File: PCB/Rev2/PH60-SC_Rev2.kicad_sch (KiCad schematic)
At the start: 43 parts, among them J1 USB_C_Receptacle_USB2.0_14P, J2 Conn_01x02_Pin, J3 Conn_01x02_Pin, U1 nRF52840, X1 32.768kHz, X2 Crystal_Generic

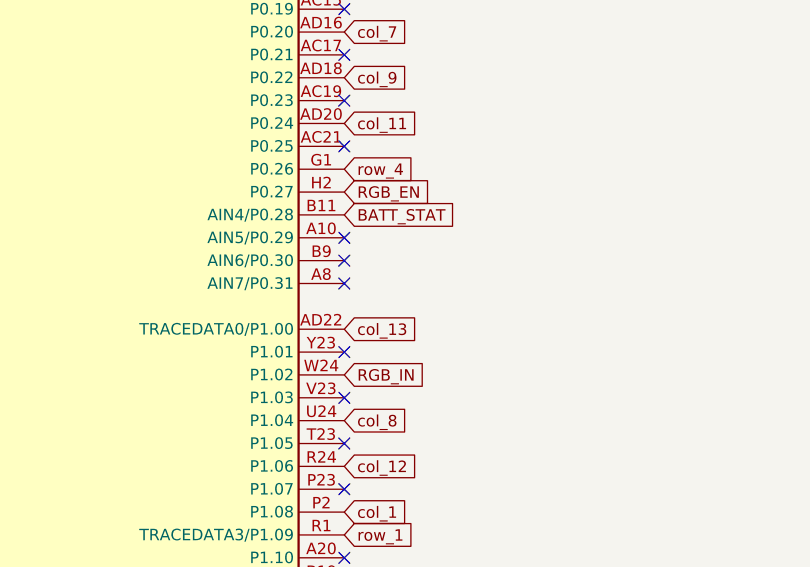
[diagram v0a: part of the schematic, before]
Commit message: layout and drc
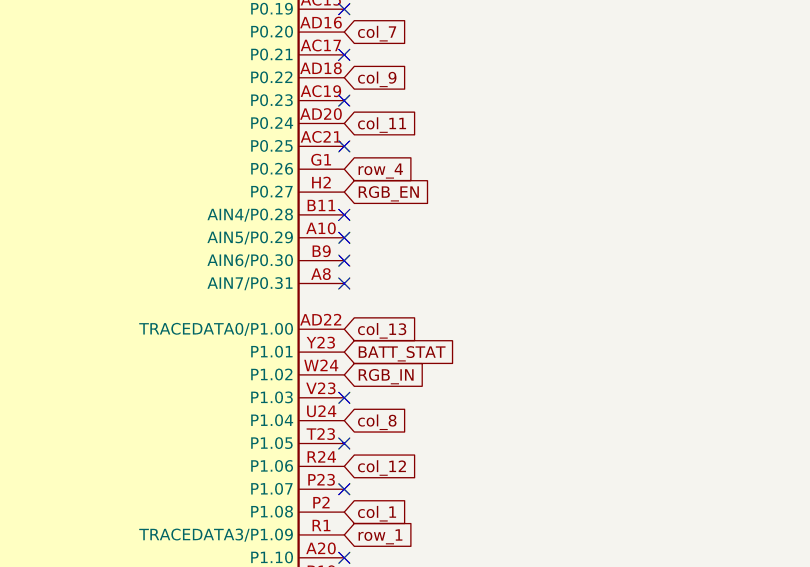
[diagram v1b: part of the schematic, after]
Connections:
- net BATT_STAT: now also U1.Y23 (P1.01); no longer U1.B11 (AIN4/P0.28)
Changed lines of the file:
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@@
+	)
+	(no_connect
+		(at 256.54 205.74)
+	)
+	(no_connect
+		(at 256.54 193.04)
+	)
+	(no_connect
+		(at 256.54 198.12)
+	)
+	(no_connect
+		(at 205.74 78.74)
+	)
+	(no_connect
+		(at 256.54 154.94)
+	)
+	(no_connect
+		(at 256.54 203.2)
+	)
+	(no_connect
+		(at 256.54 175.26)
+	)
+	(no_connect
+		(at 256.54 180.34)
+	)
+	(no_connect
+		(at 256.54 137.16)
+	)
+	(no_connect
+		(at 256.54 93.98)
 	)
 	(no_connect
@@
 	)
 	(no_connect
-		(at 256.54 205.74)
-	)
-	(no_connect
-		(at 256.54 193.04)
-	)
-	(no_connect
-		(at 256.54 198.12)
-	)
-	(no_connect
-		(at 205.74 78.74)
-	)
-	(no_connect
-		(at 256.54 203.2)
-	)
-	(no_connect
-		(at 256.54 175.26)
-	)
-	(no_connect
-		(at 256.54 180.34)
-	)
-	(no_connect
-		(at 256.54 137.16)
-	)
-	(no_connect
-		(at 256.54 93.98)
-	)
-	(no_connect
 		(at 256.54 104.14)
 	)
 	(no_connect
 		(at 256.54 99.06)
-	)
-	(no_connect
-		(at 256.54 170.18)
 	)
 	(no_connect
@@
 		)
 	)
-	(global_label "BATT_STAT"
-		(shape input)
-		(at 256.54 154.94 0)
-		(fields_autoplaced yes)
-		(effects
-			(font
-				(size 1.27 1.27)
-			)
-			(justify left)
-		)
-		(property "Intersheetrefs" "${INTERSHEET_REFS}"
-			(at 269.0199 154.94 0)
+	(global_label "RGB_EN"
+		(shape input)
+		(at 256.54 152.4 0)
+		(fields_autoplaced yes)
+		(effects
+			(font
+				(size 1.27 1.27)
+			)
+			(justify left)
+		)
+		(property "Intersheetrefs" "${INTERSHEET_REFS}"
+			(at 266.7823 152.4 0)
 			(effects
 				(font
@@
 		)
 	)
-	(global_label "RGB_EN"
-		(shape input)
-		(at 256.54 152.4 0)
-		(fields_autoplaced yes)
-		(effects
-			(font
-				(size 1.27 1.27)
-			)
-			(justify left)
-		)
-		(property "Intersheetrefs" "${INTERSHEET_REFS}"
-			(at 266.7823 152.4 0)
-			(effects
-				(font
+	(global_label "BATT_STAT"
+		(shape input)
+		(at 256.54 170.18 0)
+		(fields_autoplaced yes)
+		(effects
+			(font
+				(size 1.27 1.27)
+			)
+			(justify left)
+		)
+		(property "Intersheetrefs" "${INTERSHEET_REFS}"
+			(at 269.0199 170.18 0)
+			(effects
+				(font
